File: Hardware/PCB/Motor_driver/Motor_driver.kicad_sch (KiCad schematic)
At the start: 77 parts, among them IC1 A89307KETSR-J, J1 Conn_01x02, J2 Conn_01x05, J3 Conn_01x03, J4 629722000214, J5 USB_C_Receptacle_USB2.0_16P, J6 629712010214, SW1 SW_Push, SW3 SW_DIP_x02, SW5 SW_Push, SW6 SW_Push, U1 AZ1117-3.3, U3 STM32L412KBTx, U4 USBLC6-2SC6

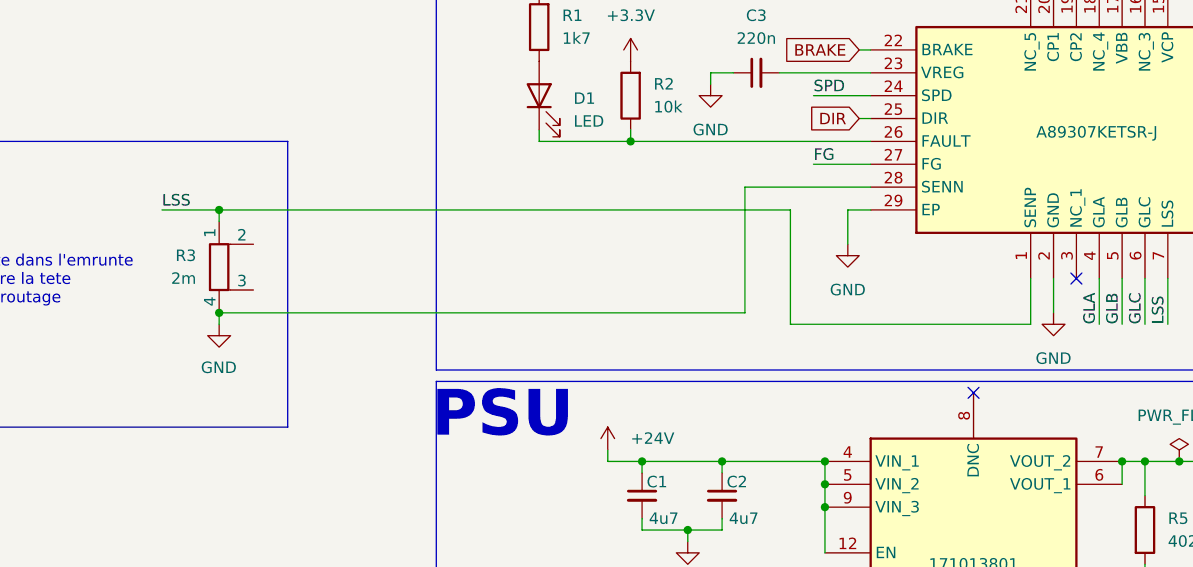
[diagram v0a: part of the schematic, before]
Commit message: Gerber
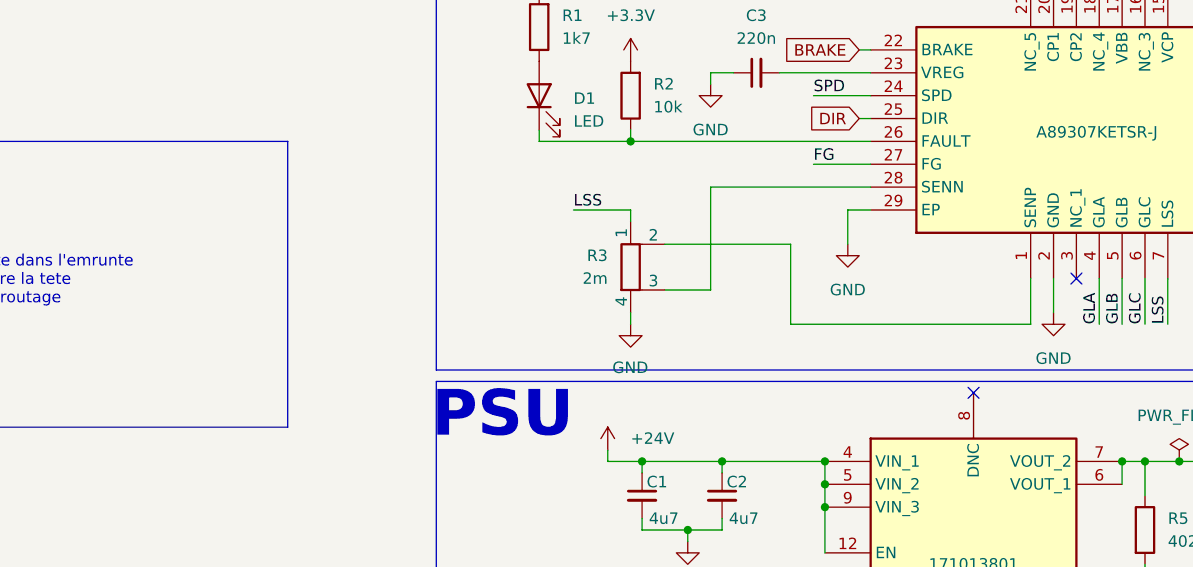
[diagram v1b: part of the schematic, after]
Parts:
- R3: footprint Resistor_SMD:R_2512_6332Metric -> Resistor_SMD:R_Shunt_Ohmite_LVK24
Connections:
- net GND: no longer IC1.28 (SENN)
- net LSS: no longer IC1.1 (SENP)
- net at R3.2: now also IC1.1 (SENP)
- net at R3.3: now also IC1.28 (SENN)
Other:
- moved on the sheet: R3
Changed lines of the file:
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@@
 	)
 	(junction
-		(at -11.43 57.15)
-		(diameter 0)
-		(color 0 0 0 0)
-	)
-	(junction
 		(at 143.51 90.17)
 		(diameter 0)
@@
 	)
 	(junction
-		(at -11.43 68.58)
-		(diameter 0)
-		(color 0 0 0 0)
-	)
-	(junction
 		(at 36.83 128.27)
 		(diameter 0)
@@
 	(wire
 		(pts
+			(xy 38.1 60.96) (xy 52.07 60.96)
+		)
+		(stroke
+			(width 0)
+			(type default)
+		)
+	)
+	(wire
+		(pts
 			(xy 232.41 38.1) (xy 245.11 38.1)
 		)
@@
 	(wire
 		(pts
+			(xy 43.18 54.61) (xy 43.18 66.04)
+		)
+		(stroke
+			(width 0)
+			(type default)
+		)
+	)
+	(wire
+		(pts
 			(xy 107.95 166.37) (xy 116.84 166.37)
 		)
@@
 	(wire
 		(pts
-			(xy 78.74 69.85) (xy 52.0433 69.85)
+			(xy 78.74 69.85) (xy 52.07 69.85)
 		)
 		(stroke
@@
 	(wire
 		(pts
-			(xy -17.78 57.15) (xy -11.43 57.15)
+			(xy 27.94 57.15) (xy 34.29 57.15)
 		)
 		(stroke
@@
 	(wire
 		(pts
-			(xy -11.43 57.15) (xy 52.0433 57.15)
-		)
-		(stroke
-			(width 0)
-			(type default)
-		)
-	)
-	(wire
-		(pts
 			(xy 251.46 140.97) (xy 251.46 142.24)
 		)
@@
 	(wire
 		(pts
-			(xy 46.99 54.61) (xy 60.96 54.61)
-		)
-		(stroke
-			(width 0)
-			(type default)
-		)
-	)
-	(wire
-		(pts
 			(xy 78.74 130.81) (xy 78.74 128.27)
 		)
@@
 	(wire
 		(pts
-			(xy 52.0433 69.85) (xy 52.0433 57.15)
+			(xy 52.07 69.85) (xy 52.07 60.96)
 		)
 		(stroke
@@
 	(wire
 		(pts
+			(xy 43.18 54.61) (xy 60.96 54.61)
+		)
+		(stroke
+			(width 0)
+			(type default)
+		)
+	)
+	(wire
+		(pts
 			(xy 229.87 100.33) (xy 229.87 97.79)
 		)
@@
 	(wire
 		(pts
-			(xy -11.43 58.42) (xy -11.43 57.15)
+			(xy 34.29 58.42) (xy 34.29 57.15)
 		)
 		(stroke
@@
 	(wire
 		(pts
+			(xy 43.18 66.04) (xy 38.1 66.04)
+		)
+		(stroke
+			(width 0)
+			(type default)
+		)
+	)
+	(wire
+		(pts
 			(xy 208.28 148.59) (xy 208.28 146.05)
 		)
@@
 	(wire
 		(pts
-			(xy 46.99 68.58) (xy 46.99 54.61)
-		)
-		(stroke
-			(width 0)
-			(type default)
-		)
-	)
-	(wire
-		(pts
 			(xy 143.51 88.9) (xy 143.51 90.17)
 		)
@@
 	(wire
 		(pts
-			(xy -11.43 68.58) (xy 46.99 68.58)
-		)
-		(stroke
-			(width 0)
-			(type default)
-		)
-	)
-	(wire
-		(pts
 			(xy 177.8 30.48) (xy 189.23 30.48)
 		)
@@
 	(wire
 		(pts
-			(xy -11.43 69.85) (xy -11.43 68.58)
+			(xy 34.29 69.85) (xy 34.29 68.58)
 		)
 		(stroke
@@
 	)
 	(label "LSS"
-		(at -17.78 57.15 0)
+		(at 27.94 57.15 0)
 		(effects
 			(font
@@
 	(symbol
 		(lib_id "Device:R_Shunt")
-		(at -11.43 63.5 0)
+		(at 34.29 63.5 0)
 		(unit 1)
 		(exclude_from_sim no)
@@
 		(fields_autoplaced yes)
 		(property "Reference" "R3"
-			(at -13.97 62.2299 0)
+			(at 31.75 62.2299 0)
 			(effects
 				(font
@@
 		)
 		(property "Value" "2m"
-			(at -13.97 64.7699 0)
+			(at 31.75 64.7699 0)
 			(effects
 				(font
@@
 			)
 		)
-		(property "Footprint" "Resistor_SMD:R_2512_6332Metric"
-			(at -13.208 63.5 90)
+		(property "Footprint" "Resistor_SMD:R_Shunt_Ohmite_LVK24"
+			(at 32.512 63.5 90)
 			(effects
 				(font
@@
 		)
 		(property "Datasheet" "~"
-			(at -11.43 63.5 0)
+			(at 34.29 63.5 0)
 			(effects
 				(font
@@
 		)
 		(property "Description" "Shunt resistor"
-			(at -11.43 63.5 0)
+			(at 34.29 63.5 0)
 			(effects
 				(font
@@
 	(symbol
 		(lib_id "power:GND")
-		(at -11.43 69.85 0)
+		(at 34.29 69.85 0)
 		(unit 1)
 		(exclude_from_sim no)
@@
 		(dnp no)
 		(property "Reference" "#PWR06"
-			(at -11.43 76.2 0)
+			(at 34.29 76.2 0)
 			(effects
 				(font
@@
 		)
 		(property "Value" "GND"
-			(at -13.462 74.676 0)
+			(at 32.258 74.676 0)
 			(effects
 				(font
@@
 		)
 		(property "Footprint" ""
-			(at -11.43 69.85 0)
+			(at 34.29 69.85 0)
 			(effects
 				(font
@@
 		)
 		(property "Datasheet" ""
-			(at -11.43 69.85 0)
+			(at 34.29 69.85 0)
 			(effects
 				(font
@@
 		)
 		(property "Description" "Power symbol creates a global label with name \"GND\" , ground"
-			(at -11.43 69.85 0)
+			(at 34.29 69.85 0)
 			(effects
 				(font
